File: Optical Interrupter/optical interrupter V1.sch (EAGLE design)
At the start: 27 parts, among them IC1 NE555, Q1 2n2222a, Q2 2n2222a, Q3 2n2222a, SW1 EC12E_SW, U1 MIC4426YN

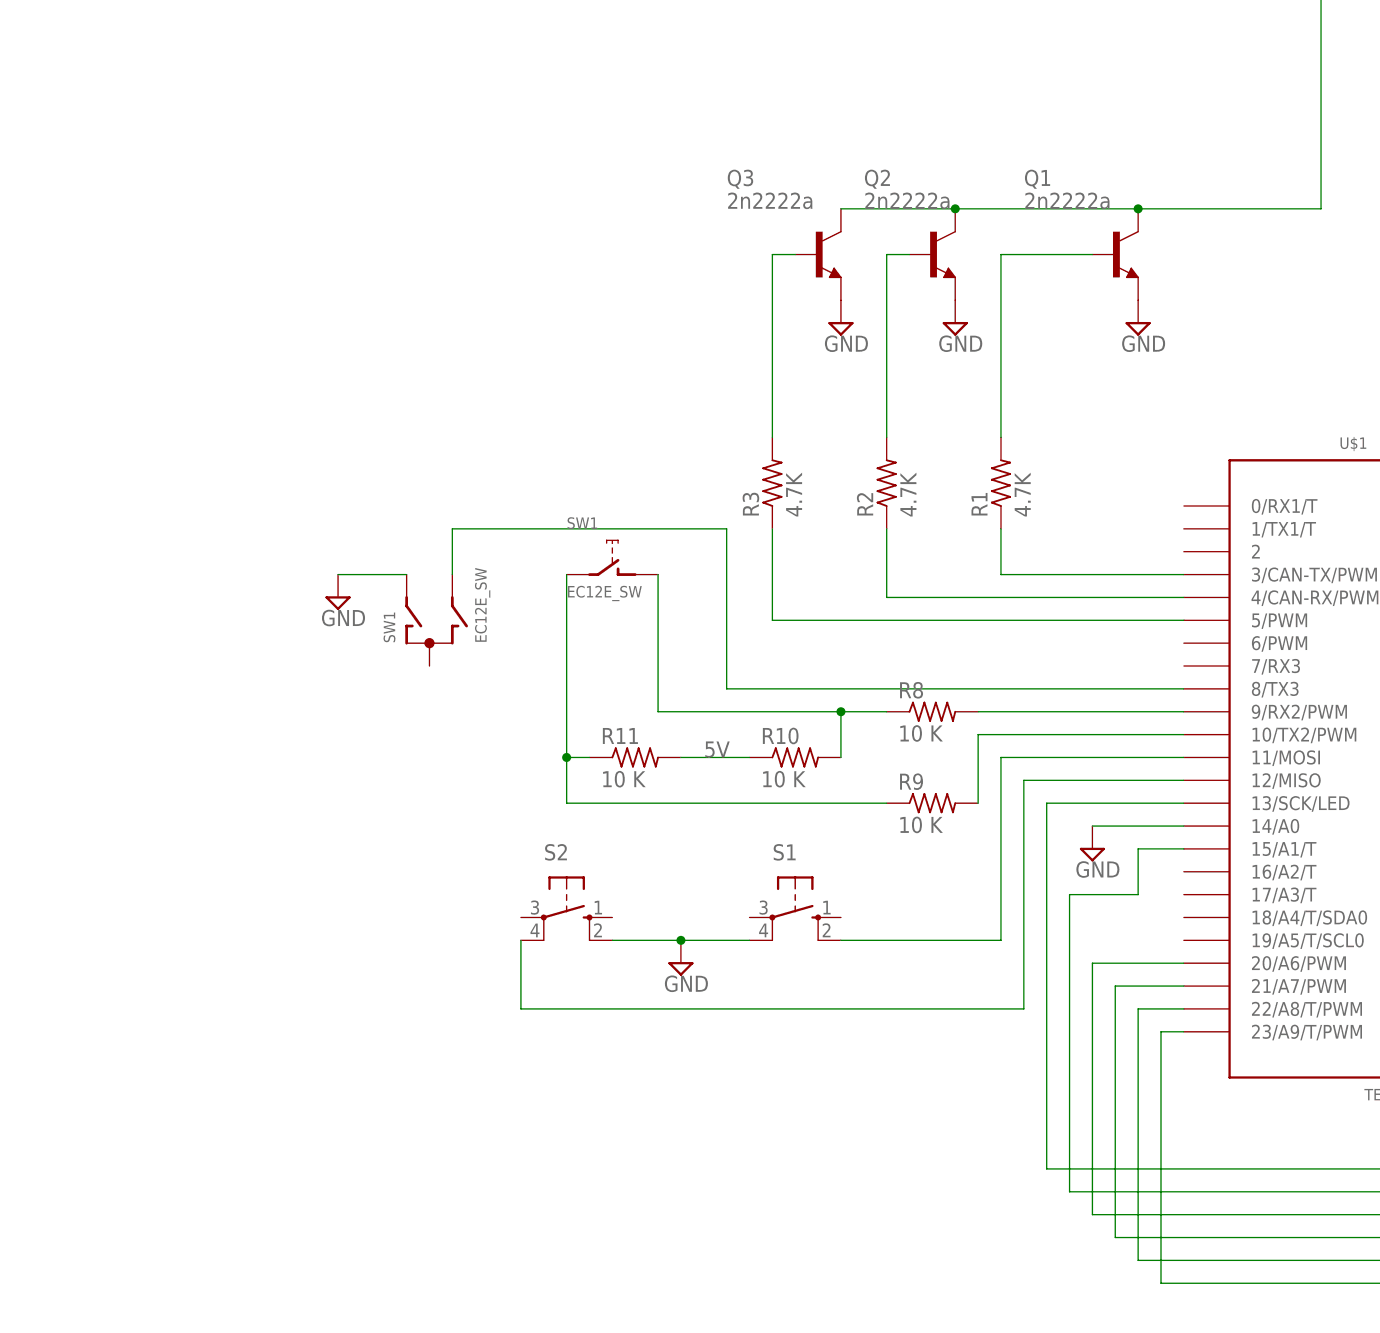
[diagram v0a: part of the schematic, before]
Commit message: updated file structure
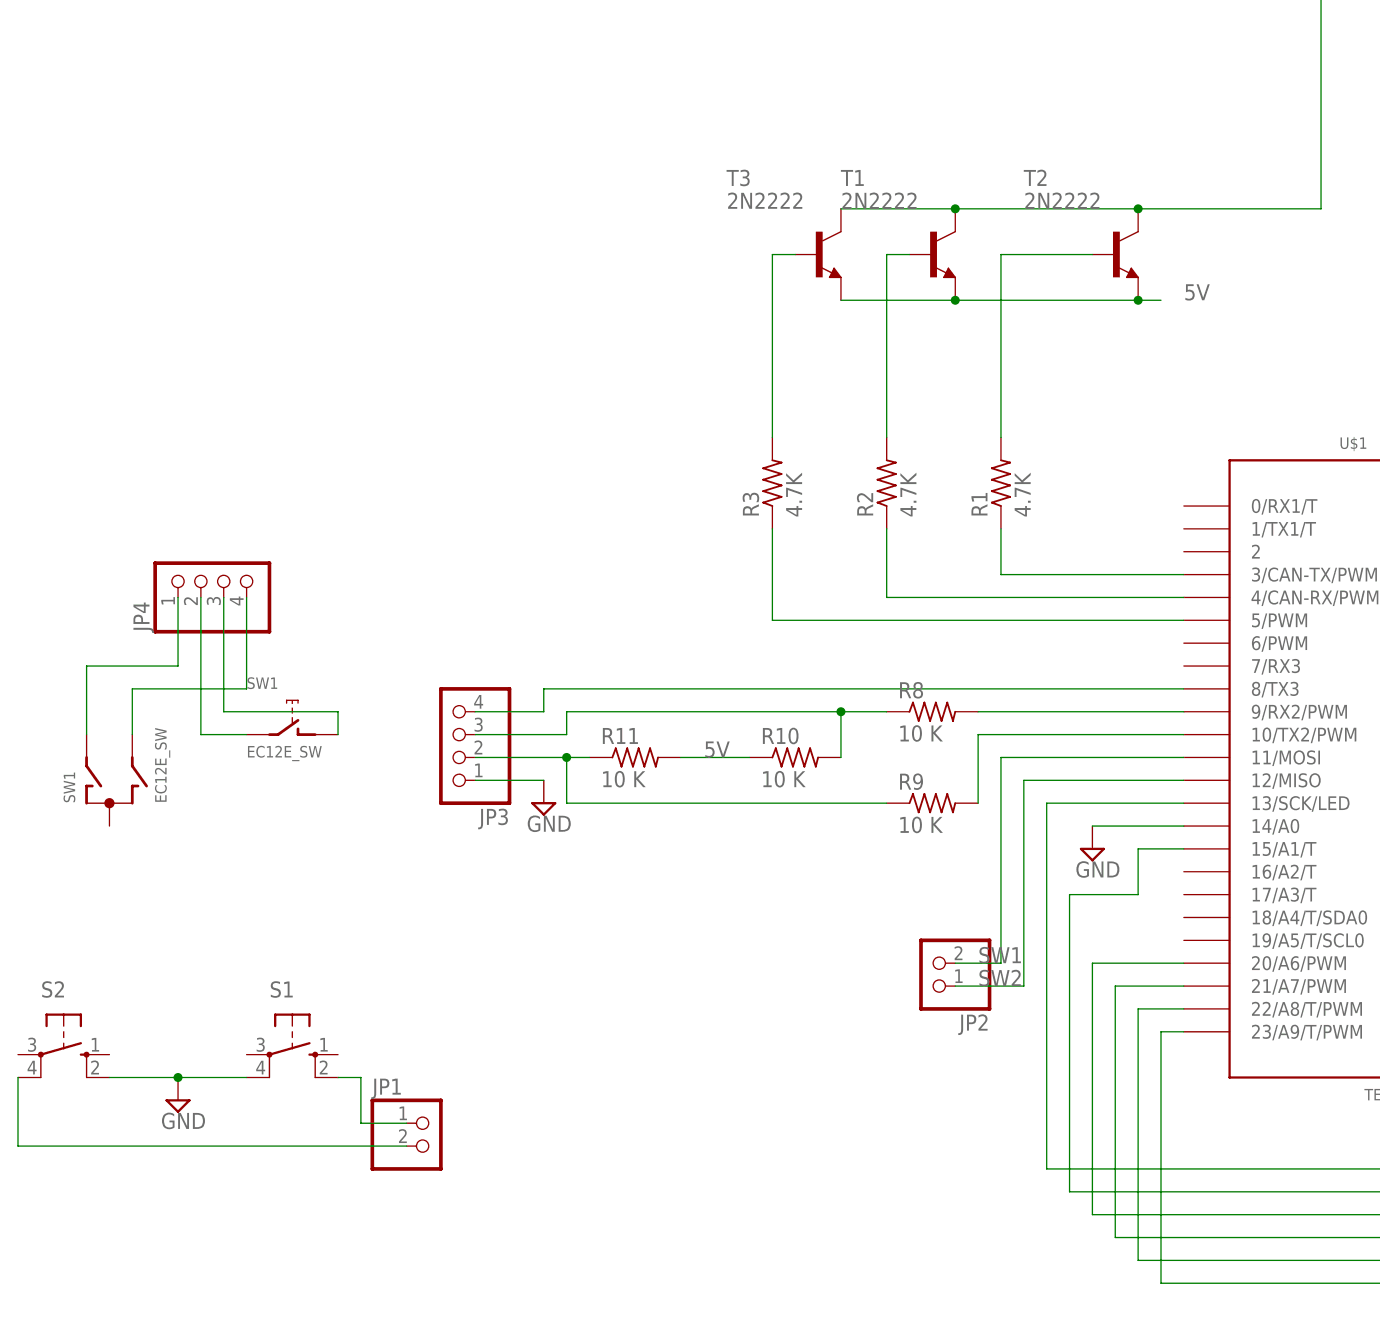
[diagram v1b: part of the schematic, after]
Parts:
- removed Q1, Q2, Q3: 2n2222a, transistor-npn:BC489
- added JP1, JP2: (no value), pinhead:PINHD-1X2
- added JP3, JP4: (no value), pinhead:PINHD-1X4
- added T1, T2, T3: 2N2222, adafruit:2N2222
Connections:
- new net N$30: JP4.1, SW1G$1.A
- new net N$31: JP4.3, SW1G$2.1
- new net N$32: JP1.1, S1.S1
- new net N$33: JP1.2, S2.P1
- new net SW1: JP2.2, U$1.11/MOSI
- new net SW2: JP2.1, U$1.12/MISO
- net 5V: now also T1.E, T2.E, T3.E
- net GND: now also JP3.1; no longer Q1.E, Q2.E, Q3.E, SW1G$1.A
- net N$14: now also JP4.2, SW1G$2.2; no longer S1.S1, U$1.11/MOSI
- net N$15: now also JP4.4, SW1G$1.B; no longer S2.P1, U$1.12/MISO
- net N$16: now also JP3.4; no longer SW1G$1.B
- net N$19: now also JP3.3; no longer SW1G$2.1
- net N$20: now also JP3.2; no longer SW1G$2.2
- net N$4: now also T2.B; no longer Q1.B
- net N$5: now also T3.B; no longer Q3.B
- net N$6: now also T1.B; no longer Q2.B
- net N$7: now also T1.C, T2.C, T3.C; no longer Q1.C, Q2.C, Q3.C
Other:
- moved on the sheet: S1, S2, SW1
